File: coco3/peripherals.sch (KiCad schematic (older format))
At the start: 61 parts, among them CN2 Conn_01x16_Female, IC14 74LS30, IC15 74LS04, IC4 W65C21N6TPLG-14, IC5 W65C21N6TPLG-14, IC7 SC77526, Q1001 MMBT9014C, U1002 MAX3232, U1003 LM393

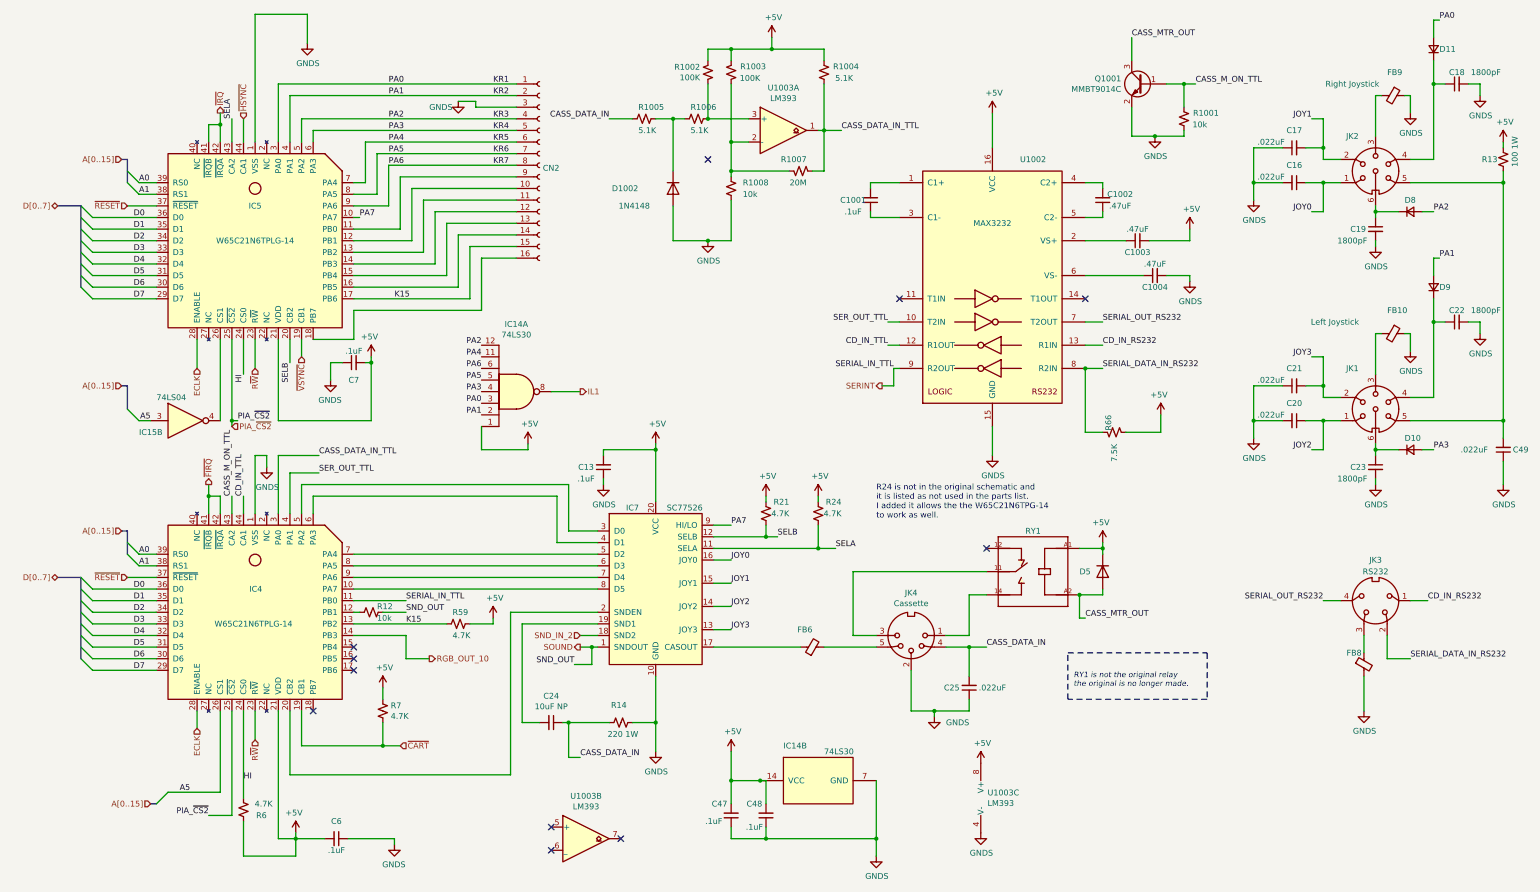
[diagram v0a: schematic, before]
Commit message: routed the board
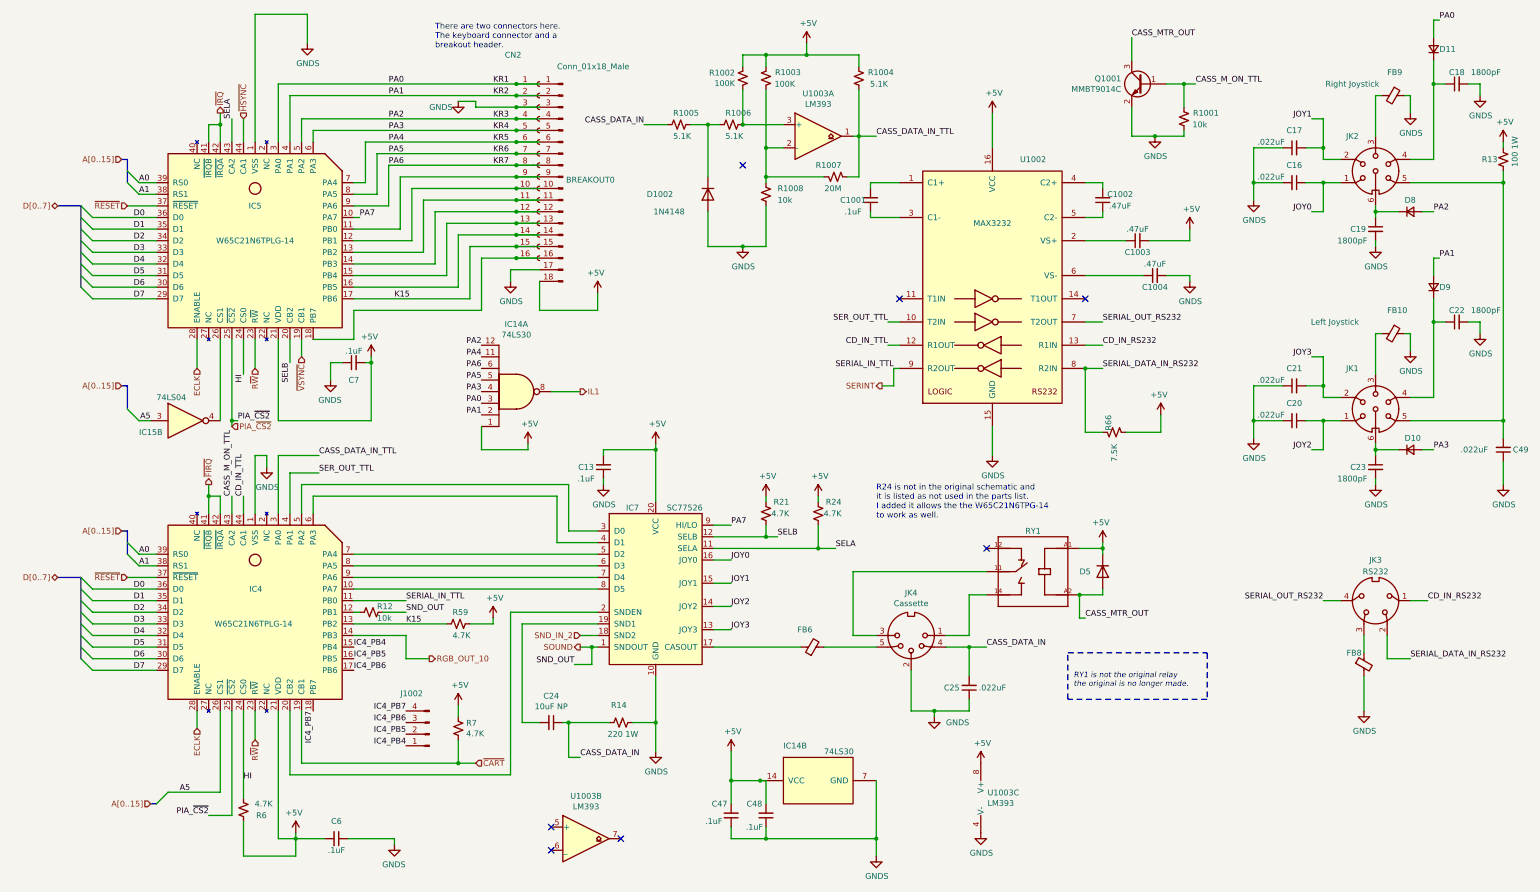
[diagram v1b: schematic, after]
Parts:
- added BREAKOUT0: Conn_01x18_Male, Connector_PinHeader_2.54mm:PinHeader_1x18_P2.54mm_Vertical, symbol Connector:Conn_01x18_Male
- added J1002: Conn_01x04_Male, Connector_PinHeader_2.54mm:PinHeader_1x04_P2.54mm_Vertical, symbol Connector:Conn_01x04_Male
- R1004, R1005, R1006: footprint Resistor_SMD:R_1206_3216Metric_Pad1.30x1.75mm_HandSolder -> Resistor_SMD:R_0805_2012Metric_Pad1.20x1.40mm_HandSolder; Manufacturer part# 1206W4F5101T5E -> 0805W8F5101T5E; Vendor part# C26033 -> C27834
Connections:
- net +5V: now also BREAKOUT0.18 (Pin_18)
- net GNDS: now also BREAKOUT0.17 (Pin_17), BREAKOUT0.3 (Pin_3)
- net K15: now also BREAKOUT0.15 (Pin_15)
- net KR1: now also BREAKOUT0.1 (Pin_1)
- net KR2: now also BREAKOUT0.2 (Pin_2)
- net KR3: now also BREAKOUT0.4 (Pin_4)
- net KR4: now also BREAKOUT0.5 (Pin_5)
- net KR5: now also BREAKOUT0.6 (Pin_6)
- net KR6: now also BREAKOUT0.7 (Pin_7)
- net KR7: now also BREAKOUT0.8 (Pin_8)
- net at CN2.10 (Pin_10), IC5.12 (PB1): now also BREAKOUT0.10 (Pin_10)
- net at CN2.11 (Pin_11), IC5.13 (PB2): now also BREAKOUT0.11 (Pin_11)
- net at CN2.12 (Pin_12), IC5.14 (PB3): now also BREAKOUT0.12 (Pin_12)
- net at CN2.13 (Pin_13), IC5.15 (PB4): now also BREAKOUT0.13 (Pin_13)
- net at CN2.14 (Pin_14), IC5.16 (PB5): now also BREAKOUT0.14 (Pin_14)
- net at CN2.16 (Pin_16), IC5.18 (PB7): now also BREAKOUT0.16 (Pin_16)
- net at CN2.9 (Pin_9), IC5.11 (PB0): now also BREAKOUT0.9 (Pin_9)
- net IC4_PB4: now reaches IC4.15 (PB4)
- net IC4_PB4: now also J1002.1 (Pin_1)
- net IC4_PB5: now reaches IC4.16 (PB5)
- net IC4_PB5: now also J1002.2 (Pin_2)
- net IC4_PB6: now reaches IC4.17 (PB6)
- net IC4_PB6: now also J1002.3 (Pin_3)
- net IC4_PB7: now reaches IC4.18 (PB7)
- net IC4_PB7: now also J1002.4 (Pin_4)
- no-connect marks 11 -> 7
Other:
- note added: "There are two connectors here.\nThe keyboard connector and a \nbreakout header."
- moved on the sheet: D1002, R1002, R1003, R1004, R1005, R1006, R1007, R1008, R7, U1003A
